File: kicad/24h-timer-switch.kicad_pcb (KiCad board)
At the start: 2 copper layers, 40.7 x 25.9 mm, 17 parts, among them J1 Barrel_Jack, J2 Screw_Terminal_01x02, Q1 FDS4559, SW1 SW_SPST, U1 AMS1117-5.0, U2 ATtiny85-20PU

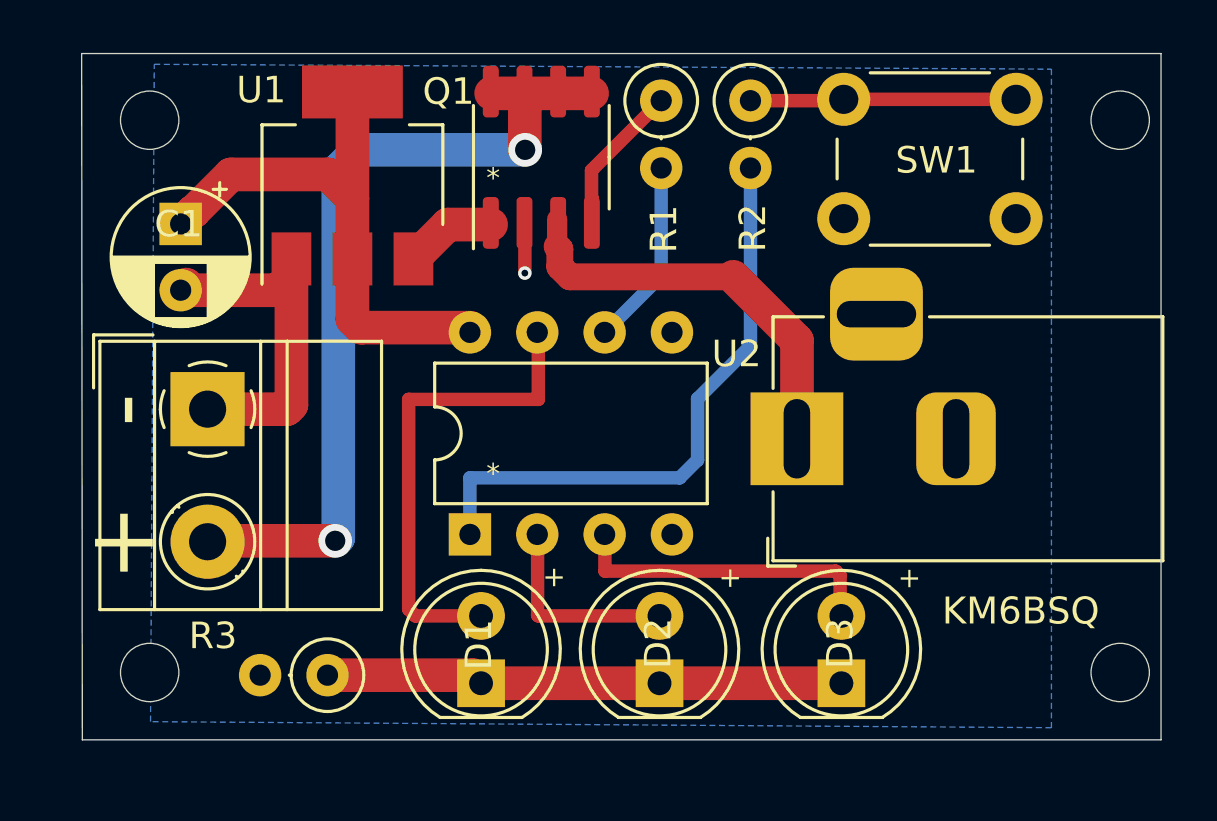
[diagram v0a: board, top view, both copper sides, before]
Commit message: full-board
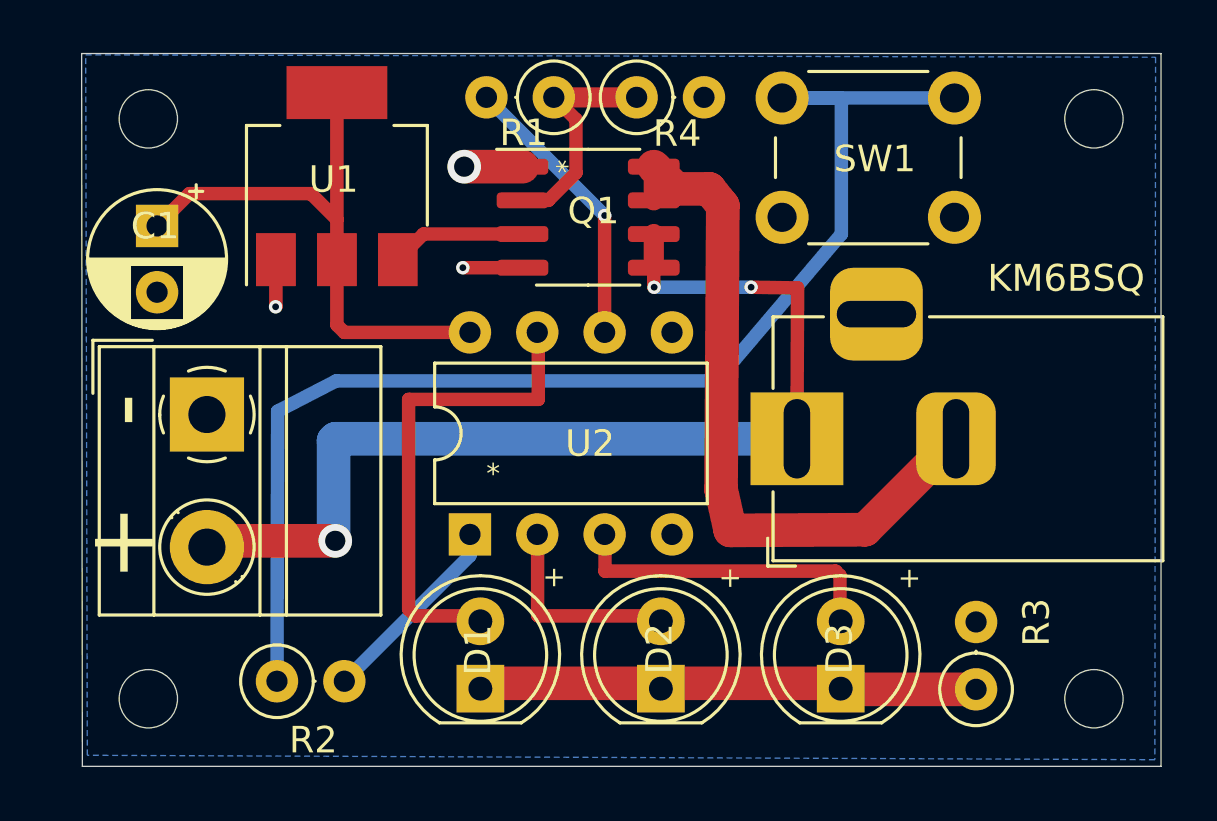
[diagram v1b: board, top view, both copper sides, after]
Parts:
- removed the REF** at (154.7, 92.7)
- removed the REF** at (154.7, 71.9)
- removed the REF** at (118.1, 71.9)
- removed the REF** at (118.1, 92.7)
- added R4: 10k, Resistor_THT:R_Axial_DIN0207_L6.3mm_D2.5mm_P2.54mm_Vertical, F.Cu at (136.5, 71.0)
- added REF**: MountingHole_2.2mm_M2, MountingHole:MountingHole_2.2mm_M2, F.Cu at (153.7, 71.8)
- added REF**: MountingHole_2.2mm_M2, MountingHole:MountingHole_2.2mm_M2, F.Cu at (118.1, 71.8)
- added REF**: MountingHole_2.2mm_M2, MountingHole:MountingHole_2.2mm_M2, F.Cu at (118.1, 93.7)
- added REF**: MountingHole_2.2mm_M2, MountingHole:MountingHole_2.2mm_M2, F.Cu at (153.7, 93.7)
- Q1: value FDS4559 -> AO4620
- moved R2 28.3 mm to (122.9, 93.0), turned to 0 degrees
- moved R3 24.5 mm to (149.3, 93.3), turned to 90 degrees
- moved R1 4.05 mm to (133.3, 71.0), turned to 180 degrees
- moved Q1 2.87 mm to (134.6, 75.5), turned to 0 degrees
- moved SW1 2.32 mm to (142.0, 71.0)
- moved C1 0.89 mm to (118.4, 75.9)
- moved U1 0.58 mm to (125.2, 74.0)
- moved D2 0.21 mm to (137.4, 93.3)
- moved J2 0.20 mm to (120.3, 83.0)
- moved D1 0.20 mm to (130.6, 93.3)
- moved D3 0.20 mm to (144.2, 93.3)
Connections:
- J1 pad 1: Net-(J1-Pad1) -> VDC
- J1 pad 2: GND -> Net-(J1-Pad2)
- Q1 pad 1: V_IN -> GND
- Q1 pad 2: GND -> Net-(Q1-Pad2)
- Q1 pad 3: Net-(J1-Pad1) -> V_IN
- Q1 pad 4: Net-(Q1-Pad4) -> GND
- Q1 pad 7: VDC -> Net-(J1-Pad2)
- Q1 pad 8: VDC -> Net-(J1-Pad2)
- R1 pad 1: Net-(Q1-Pad4) -> Net-(Q1-Pad2)
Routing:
- net Net-(R2-Pad1): track 10.0 -> 48.2 mm
- net Net-(J1-Pad2): track 0.00 -> 26.7 mm
- net Net-(J1-Pad1): track 15.6 -> 0.00 mm
- net Net-(R2-Pad2): track 22.9 -> 7.74 mm
- net GND: track 16.6 -> 6.23 mm, vias 1 -> 3
- net Net-(Q1-Pad2): track 0.00 -> 8.74 mm
- net VDC: track 32.2 -> 39.8 mm, vias 2 -> 3
- net Net-(Q1-Pad4): track 5.77 -> 0.00 mm
- net Net-(R1-Pad2): track 7.08 -> 10.7 mm, vias 0 -> 1
- net V_IN: track 3.47 -> 5.10 mm
- net VCC: track 20.8 -> 21.6 mm
- net Net-(D1-Pad1): track 19.5 -> 18.7 mm
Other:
- board size 40.7 x 25.9 mm -> 40.7 x 26.9 mm
- board text added: "24h timer switch v3"
- board text removed: "24h timer switch v1"
